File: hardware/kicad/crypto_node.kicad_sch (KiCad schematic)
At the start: 0 parts

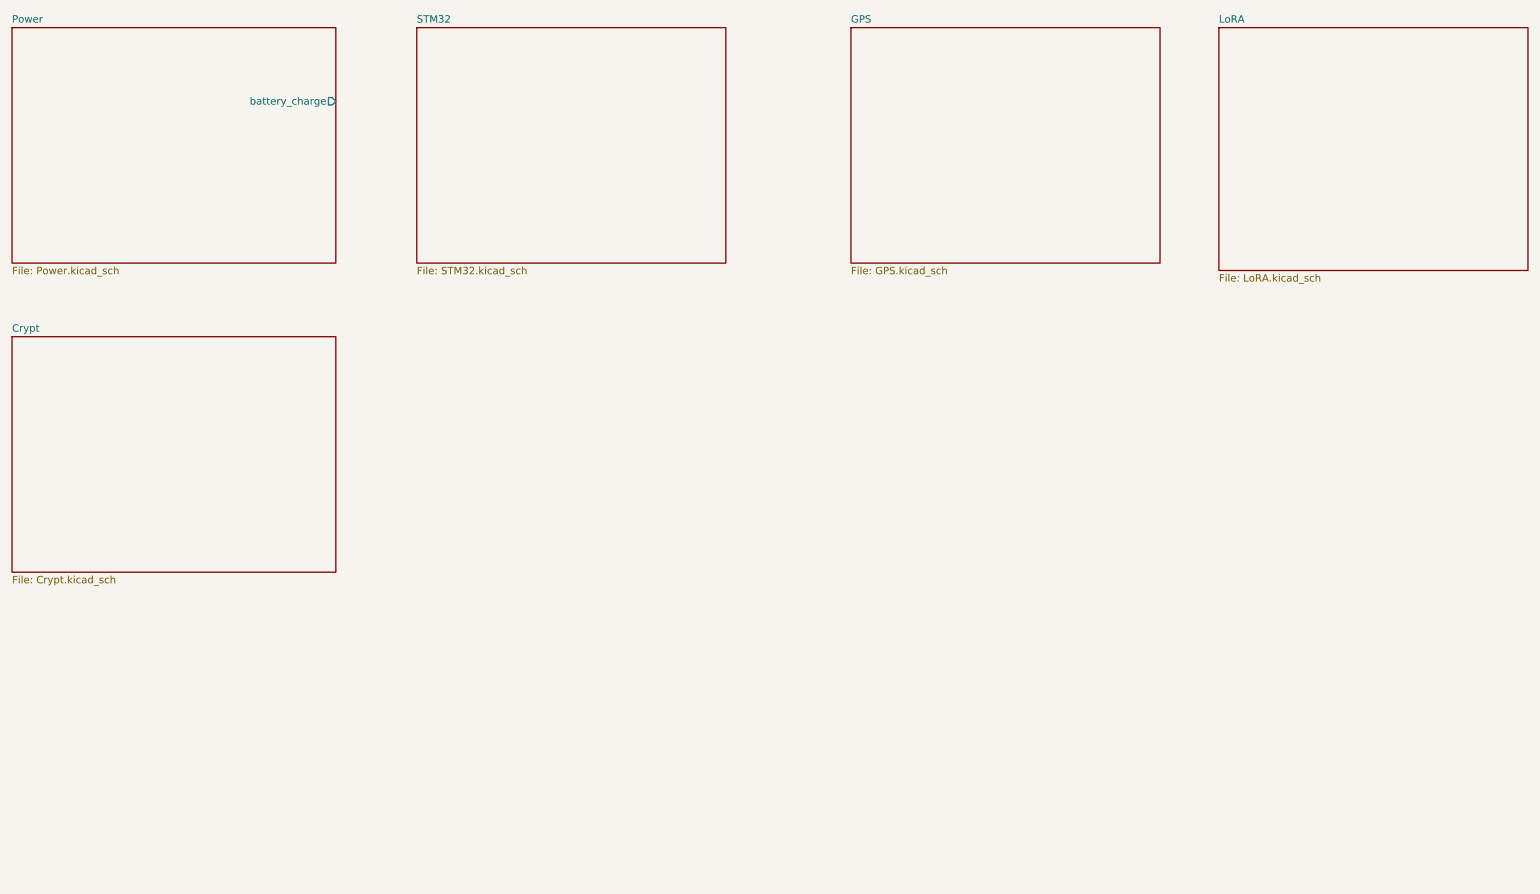
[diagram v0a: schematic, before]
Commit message: power completed
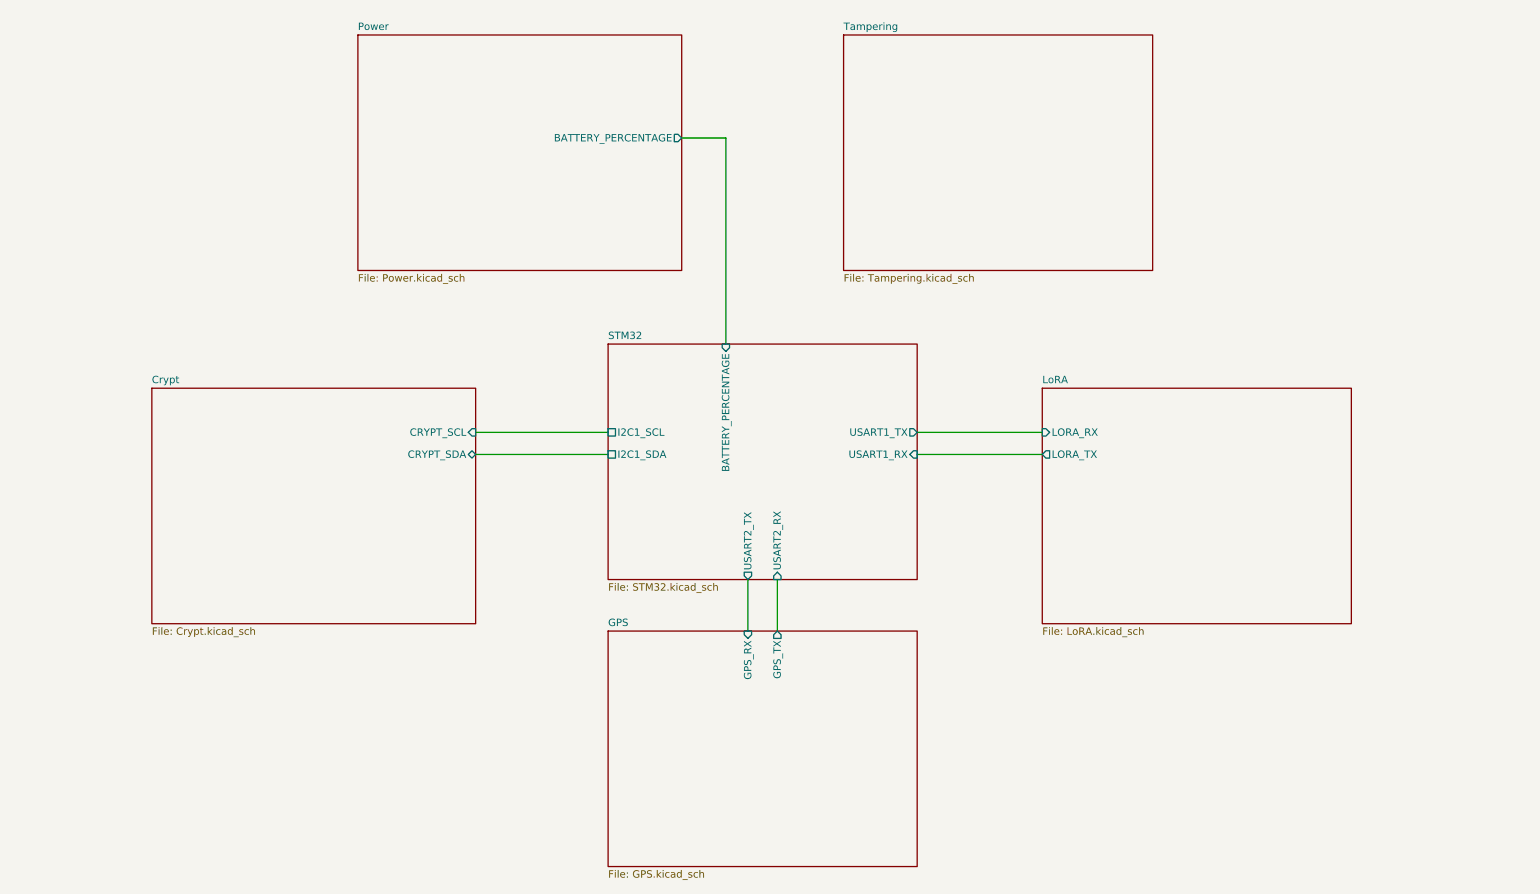
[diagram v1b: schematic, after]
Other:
- added sheet Tampering (Tampering.kicad_sch)
- sheet Crypt ports: added CRYPT_SCL, CRYPT_SDA; removed none
- sheet GPS ports: added GPS_RX, GPS_TX; removed none
- sheet LoRA ports: added LORA_RX, LORA_TX; removed none
- sheet Power ports: added BATTERY_PERCENTAGE; removed battery_charge
- sheet STM32 ports: added BATTERY_PERCENTAGE, I2C1_SCL, I2C1_SDA, USART1_RX, USART1_TX, USART2_RX, USART2_TX; removed none
